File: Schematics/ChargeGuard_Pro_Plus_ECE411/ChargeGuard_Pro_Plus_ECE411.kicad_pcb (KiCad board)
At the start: 2 copper layers, 120 x 50 mm, 25 parts, among them J1 Outlet Power (12V), J10 Solenoid, J11 Sensor Power, J12 Sensor I2C, J13 OLED Power, J14 OLED I2C, J2 Buck Converter (12V), J3 Buck Converter (5V Input), J4 Power Switch, J5 Fan, J6 Reset Switch, J7 Power Push Button, J8 Relay Module Logic, J9 Relay Module Power, Q1 2N3906, Q3 2N7000

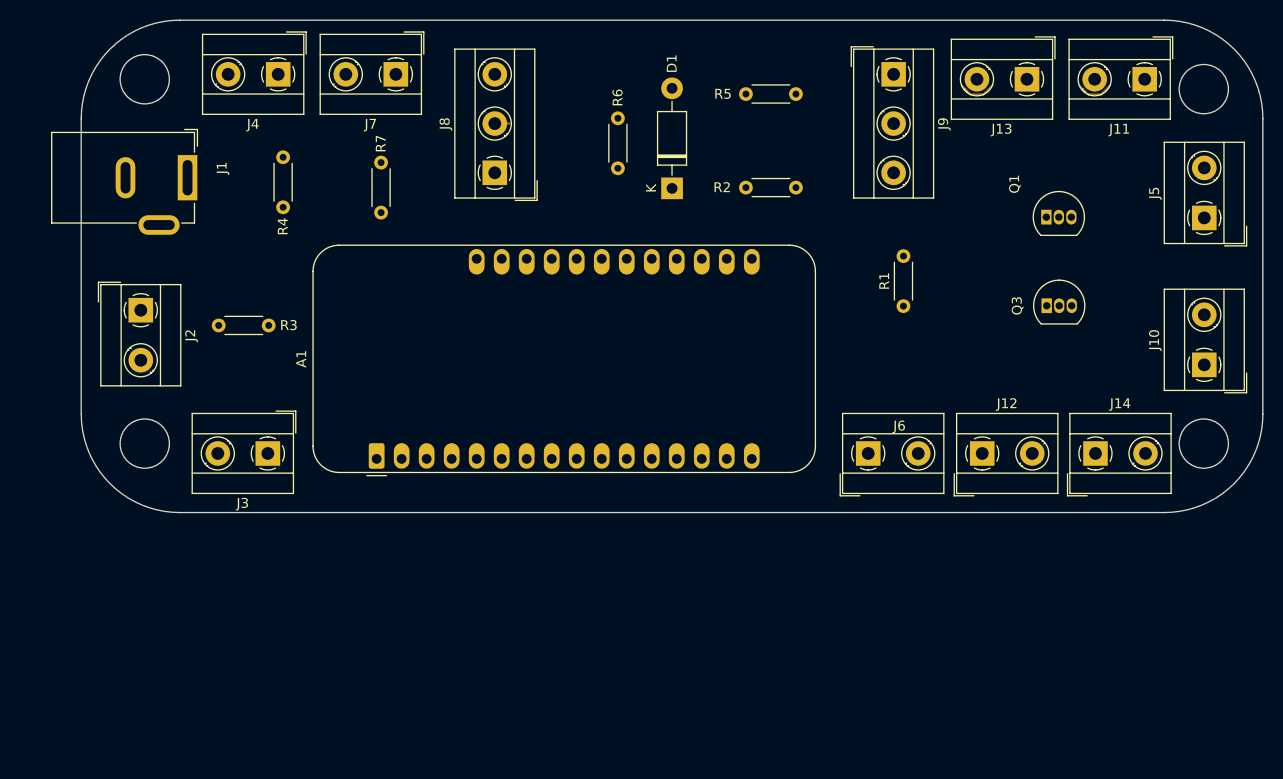
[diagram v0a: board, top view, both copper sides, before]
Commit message: ChargeGuard Pro + - 11/20/2024
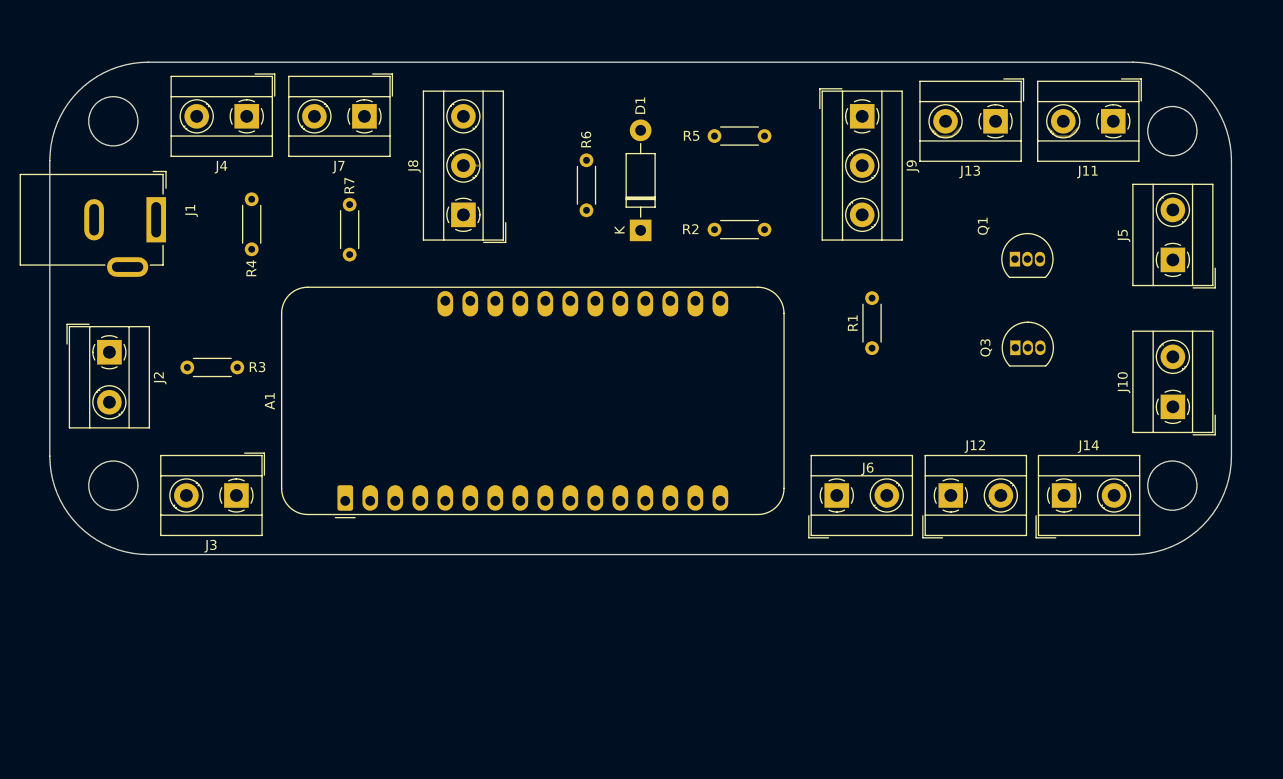
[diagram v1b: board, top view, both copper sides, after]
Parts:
- moved R7 5.33 mm to (80.2, 64.2)
- moved J3 5.33 mm to (68.7, 93.8)
- moved J7 5.33 mm to (81.7, 55.3)
- moved A1 5.33 mm to (79.8, 94.3)
- moved D1 5.33 mm to (109.8, 66.8)
- moved J1 5.33 mm to (60.6, 65.8)
- moved J10 5.33 mm to (163.8, 84.8)
- moved J11 5.33 mm to (157.8, 55.8)
- moved J12 5.33 mm to (141.3, 93.8)
- moved J13 5.33 mm to (145.8, 55.8)
- moved J14 5.33 mm to (152.8, 93.8)
- moved J2 5.33 mm to (55.8, 79.2)
- moved J4 5.33 mm to (69.8, 55.3)
- moved J5 5.33 mm to (163.8, 69.8)
- moved J6 5.33 mm to (129.7, 93.8)
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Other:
- outline, holes or cut-outs redrawn
- board text added: "0.0000 mm / 0.0000 mm"
- board text added: "0.3000 mm"
- board text added: "1.6000 mm"
- board text added: "120.0000 mm x 50.0000 mm"
- board text added: "2"
- board text added: "BOARD CHARACTERISTICS"
- board text added: "Board Thickness:"
- board text added: "Board overall dimensions:"
- board text added: "Castellated pads:"
- board text added: "ChargeGuard Pro + PSU - ECE411 - Team #2 Fall 2024"
- board text added: "Copper Finish:"
- board text added: "Copper Layer Count:"
- board text added: "Edge card connectors:"
- board text added: "Impedance Control:"
- board text added: "Min hole diameter:"
- board text added: "Min track/spacing:"
- board text added: "No"
- board text added: "None"
- board text added: "Plated Board Edge:"

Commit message: ChargeGuard Pro +  - 11/21/2024
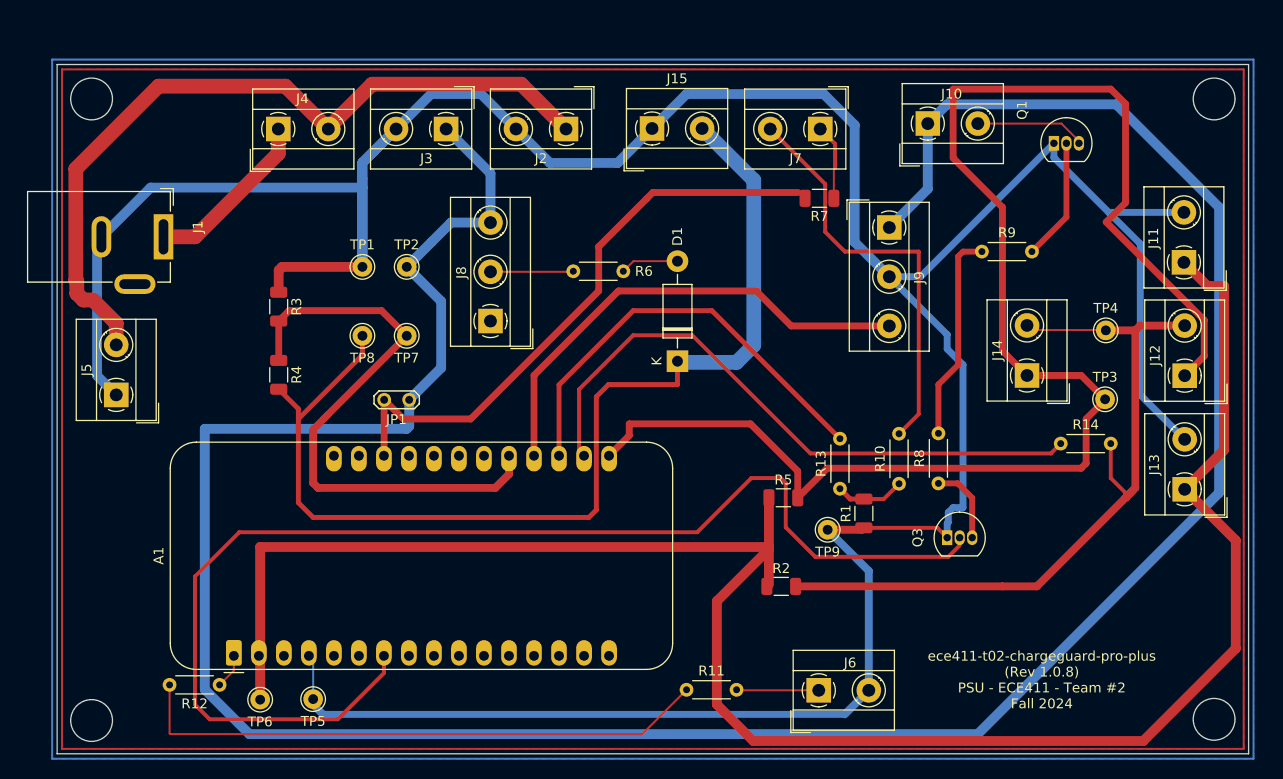
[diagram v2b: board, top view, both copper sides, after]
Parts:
- added J15: Battery, TerminalBlock_MetzConnect:TerminalBlock_MetzConnect_Type101_RT01602HBWC_1x02_P5.08mm_Horizontal, F.Cu at (110.9, 56.5)
- added JP1: Protection jumper, TestPoint:TestPoint_2Pads_Pitch2.54mm_Drill0.8mm, F.Cu at (86.3, 84.1)
- added R10: 0, Resistor_THT:R_Axial_DIN0204_L3.6mm_D1.6mm_P5.08mm_Horizontal, F.Cu at (136.0, 92.6)
- added R11: 0, Resistor_THT:R_Axial_DIN0204_L3.6mm_D1.6mm_P5.08mm_Horizontal, F.Cu at (114.4, 113.5)
- added R12: 0, Resistor_THT:R_Axial_DIN0204_L3.6mm_D1.6mm_P5.08mm_Horizontal, F.Cu at (67.0, 113.0)
- added R13: 0, Resistor_THT:R_Axial_DIN0204_L3.6mm_D1.6mm_P5.08mm_Horizontal, F.Cu at (130.0, 93.1)
- added R14: 0, Resistor_THT:R_Axial_DIN0204_L3.6mm_D1.6mm_P5.08mm_Horizontal, F.Cu at (152.4, 88.5)
- added R8: 0, Resistor_THT:R_Axial_DIN0204_L3.6mm_D1.6mm_P5.08mm_Horizontal, F.Cu at (140.0, 92.5)
- added R9: 0, Resistor_THT:R_Axial_DIN0204_L3.6mm_D1.6mm_P5.08mm_Horizontal, F.Cu at (144.4, 69.0)
- added TP1: 5V(-), Connector_Pin:Pin_D1.0mm_L10.0mm, F.Cu at (81.5, 70.6)
- added TP2: 5V(+), Connector_Pin:Pin_D1.0mm_L10.0mm, F.Cu at (86.0, 70.6)
- added TP3: SDA, Connector_Pin:Pin_D1.0mm_L10.0mm, F.Cu at (156.9, 84.0)
- added TP4: SCL, Connector_Pin:Pin_D1.0mm_L10.0mm, F.Cu at (157.0, 77.0)
- added TP5: GND, Connector_Pin:Pin_D1.0mm_L10.0mm, F.Cu at (76.5, 114.4)
- added TP6: 3.3V, Connector_Pin:Pin_D1.0mm_L10.0mm, F.Cu at (71.1, 114.5)
- added TP7: VD, Connector_Pin:Pin_D1.0mm_L10.0mm, F.Cu at (86.0, 77.6)
- added TP8: BAT, Connector_Pin:Pin_D1.0mm_L10.0mm, F.Cu at (81.5, 77.6)
- added TP9: Via, Connector_Pin:Pin_D1.0mm_L10.0mm, F.Cu at (128.8, 97.2)
- J1: value Outlet Power (12V) -> Barrel_Jack_MountingPin
- J3: value Buck Converter (5V Input) -> Buck Converter (5V output)
- J7: value Power Push Button -> Power PB
- R1, R2, R4, R5, R7: footprint Resistor_THT:R_Axial_DIN0204_L3.6mm_D1.6mm_P5.08mm_Horizontal -> Resistor_SMD:R_1206_3216Metric
- R3: value 1k -> 8.2k; footprint Resistor_THT:R_Axial_DIN0204_L3.6mm_D1.6mm_P5.08mm_Horizontal -> Resistor_SMD:R_1206_3216Metric
- moved J5 108.2 mm to (56.5, 83.6)
- moved J2 51.6 mm to (102.2, 56.5), turned to 180 degrees
- moved R7 47.7 mm to (127.9, 63.6), turned to 180 degrees
- moved J7 46.3 mm to (128.0, 56.6)
- moved J3 42.9 mm to (90.0, 56.6)
- moved J13 42.0 mm to (165.0, 93.1), turned to 90 degrees
- moved J10 38.0 mm to (138.9, 56.0), turned to 0 degrees
- moved R5 36.8 mm to (124.2, 94.0), turned to 0 degrees
- moved R2 36.3 mm to (124.0, 103.0), turned to 0 degrees
- moved J12 26.7 mm to (165.0, 81.6), turned to 90 degrees
- moved Q3 20.5 mm to (140.9, 98.1)
- moved J6 19.9 mm to (127.8, 113.6)
- moved A1 19.4 mm to (68.5, 110.1)
- moved R4 18.0 mm to (73.0, 81.5)
- moved R1 16.8 mm to (132.4, 95.6)
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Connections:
- net Battery terminal (AA+) renamed Net-(D1-K)
- A1 pad 26: Power (Buck Converter '+') -> Net-(A1-USB)
- A1 pad 4: Battery Terminal (AA-) -> GND
- J1 pad 2: Net-(J2-Pin_2) -> GND
- J11 pad 1: Battery Terminal (AA-) -> I2C Power
- J11 pad 2: Power (Buck Converter '+') -> GND
- J12 pad 2: Net-(A1-SCL/IO22) -> Net-(J12-Pin_2)
- J13 pad 1: Battery Terminal (AA-) -> I2C Power
- J13 pad 2: Power (Buck Converter '+') -> GND
- J14 pad 2: Net-(A1-SCL/IO22) -> Net-(J12-Pin_2)
- J2 pad 2: Net-(J2-Pin_2) -> GND
- J3 pad 2: Battery Terminal (AA-) -> GND
- J5 pad 1: Net-(J2-Pin_2) -> GND
- J6 pad 1: Net-(A1-~{RESET}) -> Net-(J6-Pin_1)
- J6 pad 2: Battery Terminal (AA-) -> GND
- J7 pad 2: Net-(A1-A6/IO14) -> Net-(J7-Pin_2)
- J9 pad 2: Battery Terminal (AA-) -> GND
- Q1 pad 1: Battery Terminal (AA-) -> GND
- Q3 pad 1: Battery Terminal (AA-) -> GND
- Q3 pad 3: Net-(Q1-B) -> Net-(Q3-D)
- R1 pad 1: Battery Terminal (AA-) -> GND
- R1 pad 2: Net-(A1-A6/IO14) -> Net-(R1-Pad2)
- R2 pad 2: Net-(A1-SCL/IO22) -> Net-(J12-Pin_2)
- R3 pad 1: Battery Terminal (AA-) -> GND
- R7 pad 2: Power (Buck Converter '+') -> Net-(A1-USB)
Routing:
- net GND: track 0.00 -> 350.5 mm
- net Power (Buck Converter '+'): track 0.07 -> 279.5 mm
- net I2C Power: track 0.00 -> 199.0 mm
- net Net-(A1-SDA/IO23): track 0.00 -> 156.5 mm
- net Net-(A1-I34/A2): track 0.00 -> 125.5 mm
- net Net-(D1-K): track 0.00 -> 110.0 mm
- net Net-(J2-Pin_1): track 0.00 -> 79.0 mm
- net Net-(J12-Pin_2): track 0.00 -> 78.7 mm
- net Net-(A1-SCL/IO22): track 0.00 -> 63.5 mm
- net Net-(A1-USB): track 0.00 -> 61.6 mm
- net Net-(A1-A8/IO15): track 0.00 -> 60.6 mm
- net Net-(R11-Pad1): track 0.00 -> 59.3 mm
- net Net-(A1-A7/IO32): track 0.00 -> 49.3 mm
- net Net-(A1-A6/IO14): track 0.00 -> 44.2 mm
- net Net-(J7-Pin_2): track 0.00 -> 42.4 mm
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- added copper zone on B.Cu, net (none)
- added copper zone on F.Cu, net Power (Buck Converter '+')
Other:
- board size 120 x 50 mm -> 121 x 70 mm
- board text added: "ece411-t02-chargeguard-pro-plus (Rev 1.0.8) PSU - ECE411 - Team #2 Fall 2024"
- board text removed: "0.0000 mm / 0.0000 mm"
- board text removed: "0.3000 mm"
- board text removed: "1.6000 mm"
- board text removed: "120.0000 mm x 50.0000 mm"
- board text removed: "2"
- board text removed: "BOARD CHARACTERISTICS"
- board text removed: "Board Thickness:"
- board text removed: "Board overall dimensions:"
- board text removed: "Castellated pads:"
- board text removed: "ChargeGuard Pro + PSU - ECE411 - Team #2 Fall 2024"
- board text removed: "Copper Finish:"
- board text removed: "Copper Layer Count:"
- board text removed: "Edge card connectors:"
- board text removed: "Impedance Control:"
- board text removed: "Min hole diameter:"
- board text removed: "Min track/spacing:"
- board text removed: "No"
- board text removed: "None"
- board text removed: "Plated Board Edge:"
